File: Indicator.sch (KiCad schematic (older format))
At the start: 17 parts, among them U10 BC56-12SURKWA, U11 SC56-11SRWA, U12 MAX7219EWG+T, U8 CC56-12SURKWA, U9 MAX7219EWG+T

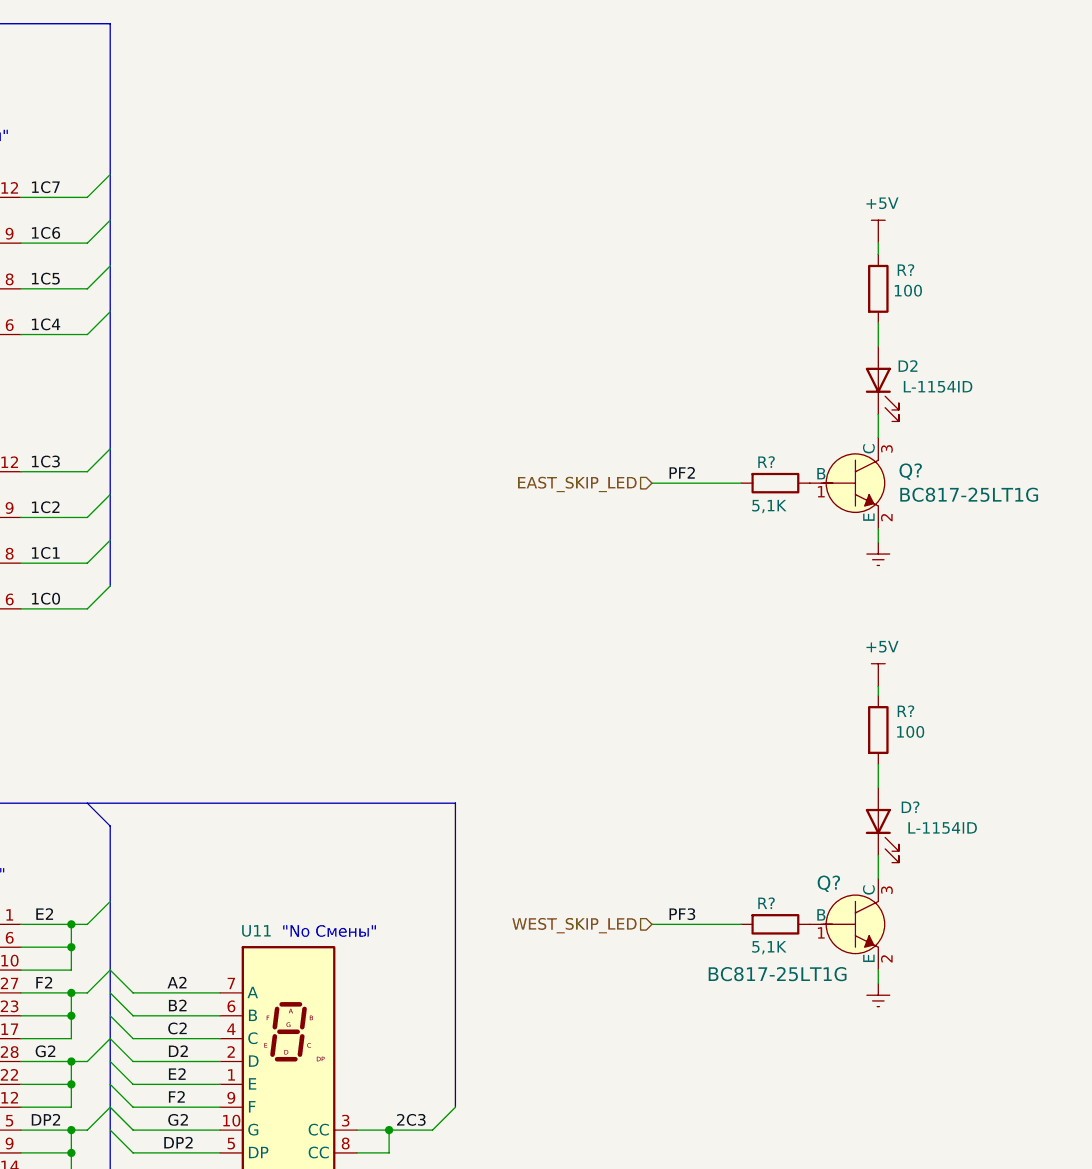
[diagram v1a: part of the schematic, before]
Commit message: Digital IO ended
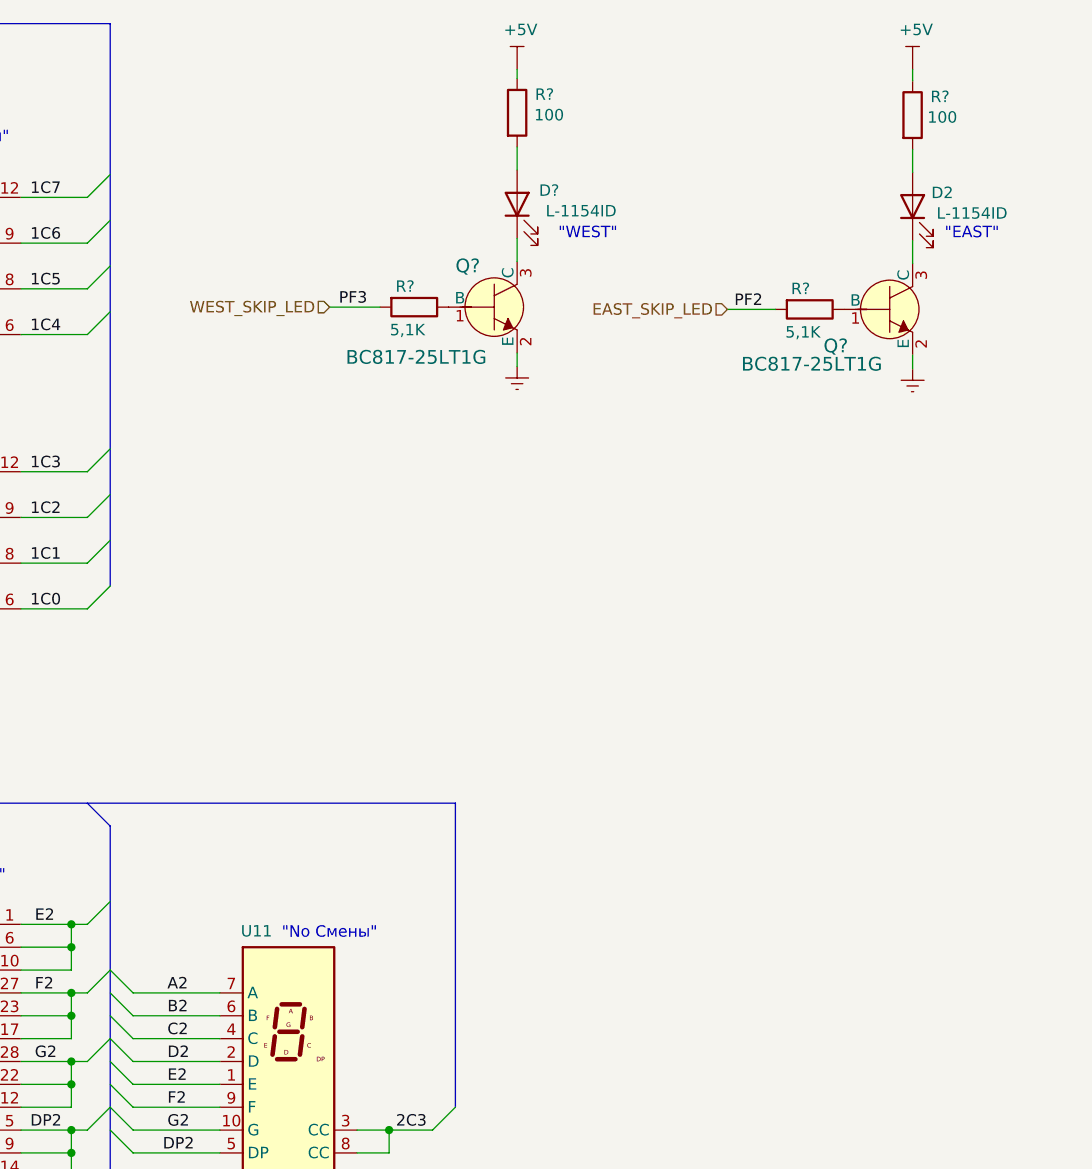
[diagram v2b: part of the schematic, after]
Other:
- note added: ""EAST""
- note added: ""WEST""
- moved on the sheet: D2, D?, Q?, R?
